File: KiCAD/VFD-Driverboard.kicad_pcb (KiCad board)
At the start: 2 copper layers, 100 x 20.5 mm, 16 parts, among them U1 MC34063AD, U2 LM4871MX_NOPB

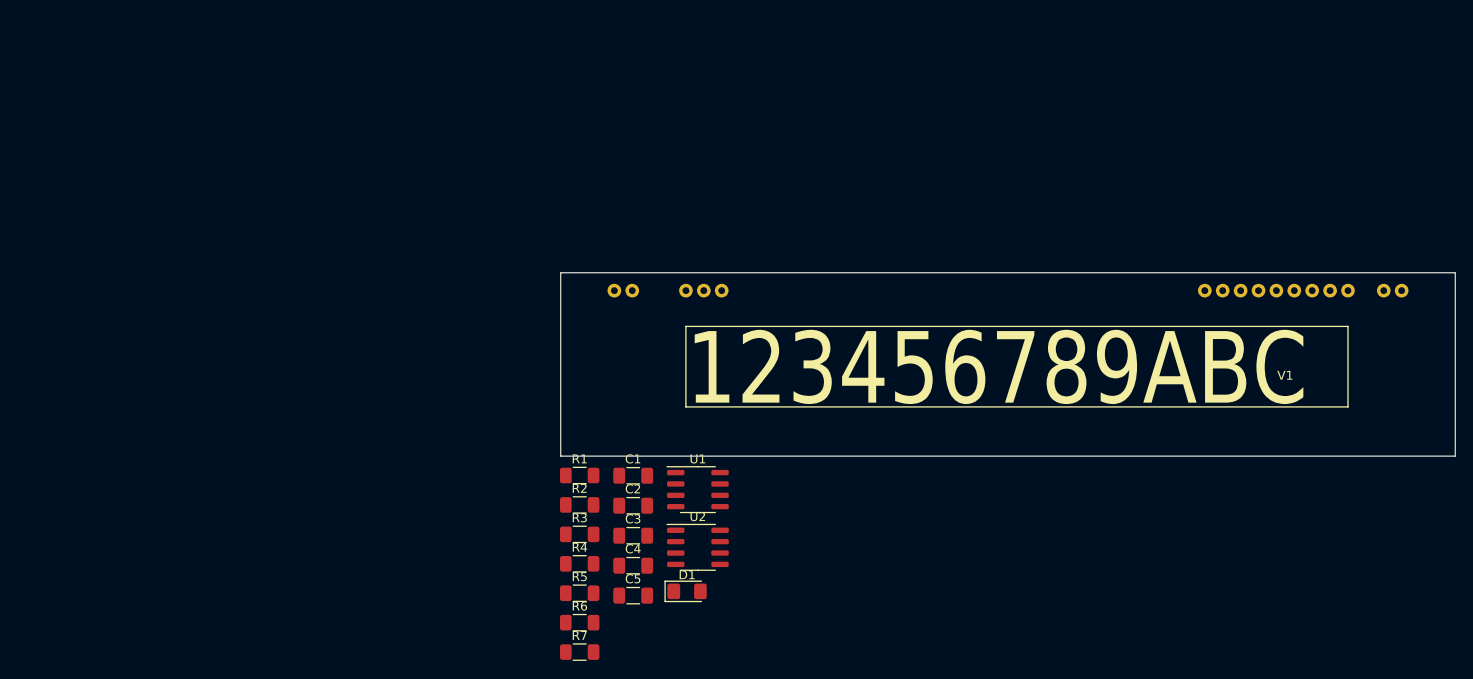
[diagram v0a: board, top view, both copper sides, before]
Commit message: Driverboard v. 1.0.4
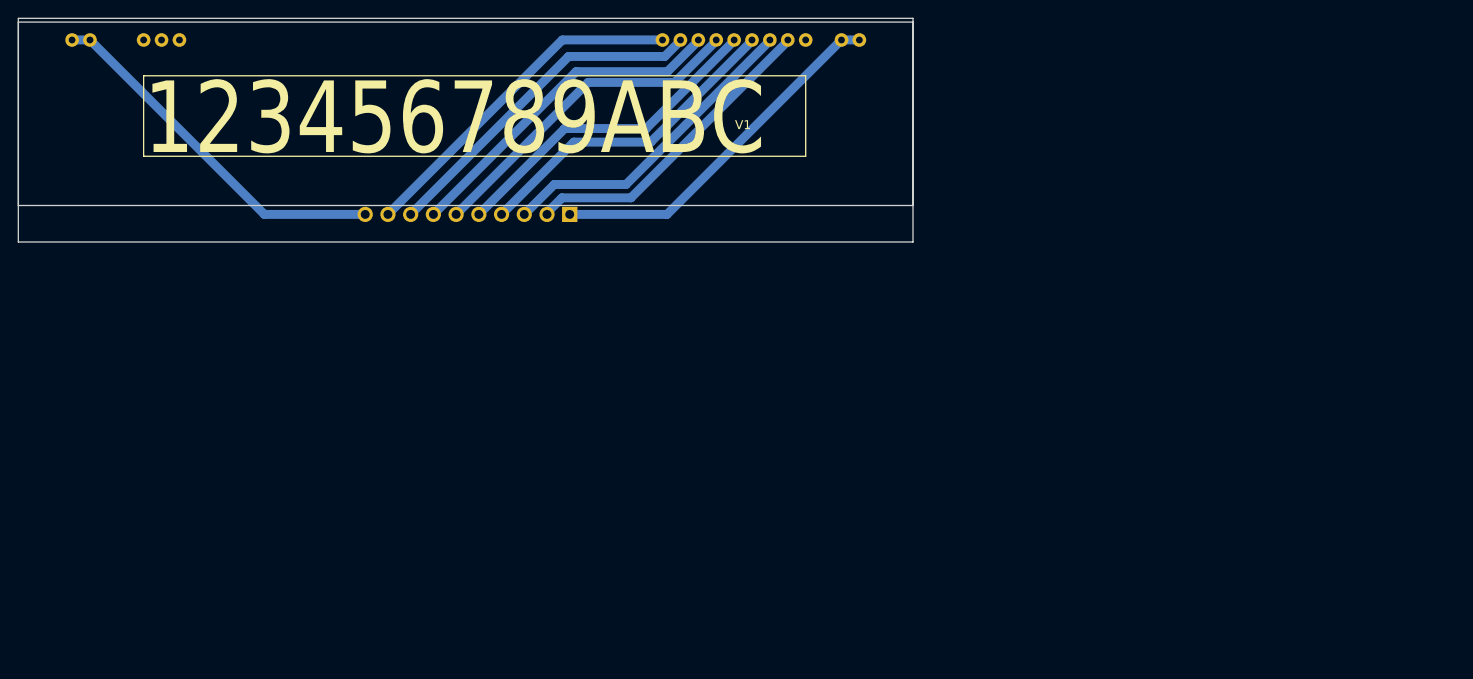
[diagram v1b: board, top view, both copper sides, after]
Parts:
- removed C1, C3, C4, C5: 1u, Capacitor_SMD:C_1206_3216Metric_Pad1.33x1.80mm_HandSolder
- removed C2: 10n, Capacitor_SMD:C_1206_3216Metric_Pad1.33x1.80mm_HandSolder
- removed D1: 2V7, Diode_SMD:D_1206_3216Metric_Pad1.42x1.75mm_HandSolder
- removed R1, R2, R4: 10k, Resistor_SMD:R_1206_3216Metric_Pad1.30x1.75mm_HandSolder
- removed R3: 2k2, Resistor_SMD:R_1206_3216Metric_Pad1.30x1.75mm_HandSolder
- removed R5, R6: 1k, Resistor_SMD:R_1206_3216Metric_Pad1.30x1.75mm_HandSolder
- removed R7: R, Resistor_SMD:R_1206_3216Metric_Pad1.30x1.75mm_HandSolder
- removed U1: MC34063AD, Package_SO:SOIC-8_3.9x4.9mm_P1.27mm
- removed U2: LM4871MX_NOPB, Package_SO:SOIC-8_3.9x4.9mm_P1.27mm
- added J2: Breadboard, Connector_PinHeader_2.54mm:PinHeader_1x10_P2.54mm_Vertical, B.Cu at (75.0, 35.3)
- moved V1 66.8 mm to (13.3, 14.0)
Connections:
- V1 pad 10: unconnected-(V1-CS-Pad10) -> Net-(J1-Pin_6)
- V1 pad 11: unconnected-(V1-Clk-Pad11) -> Net-(J1-Pin_7)
- V1 pad 12: unconnected-(V1-DI-Pad12) -> Net-(J1-Pin_8)
- V1 pad 5: unconnected-(V1-VDD-Pad5) -> VCC
- V1 pad 7: unconnected-(V1-Gnd-Pad7) -> GNDD
- V1 pad 8: unconnected-(V1-OSC0-Pad8) -> Net-(J1-Pin_4)
- V1 pad 9: unconnected-(V1-Reset-Pad9) -> Net-(J1-Pin_5)
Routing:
- net VF2: track 0.00 -> 40.8 mm
- net VF1: track 0.00 -> 40.4 mm
- net Net-(J1-Pin_8): track 0.00 -> 38.8 mm
- net Net-(J1-Pin_7): track 0.00 -> 38.3 mm
- net Net-(J1-Pin_6): track 0.00 -> 37.7 mm
- net Net-(J1-Pin_5): track 0.00 -> 37.2 mm
- net Net-(J1-Pin_4): track 0.00 -> 36.7 mm
- net GNDD: track 0.00 -> 36.1 mm
- net VEE: track 0.00 -> 35.6 mm
- net VCC: track 0.00 -> 35.2 mm
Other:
- board size 100 x 20.5 mm -> 100 x 25 mm
